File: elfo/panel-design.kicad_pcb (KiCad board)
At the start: 2 copper layers, 20 x 128.3 mm, 16 parts

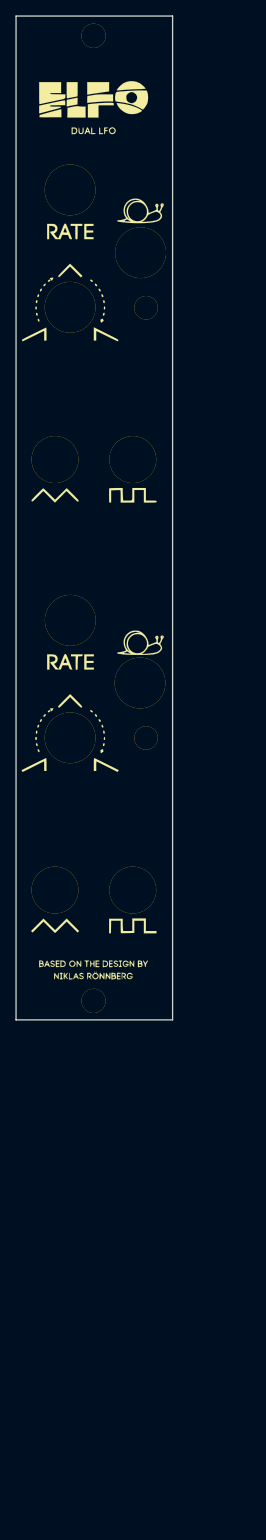
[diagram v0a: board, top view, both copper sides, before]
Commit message: Make ELFO nicer, fix issues
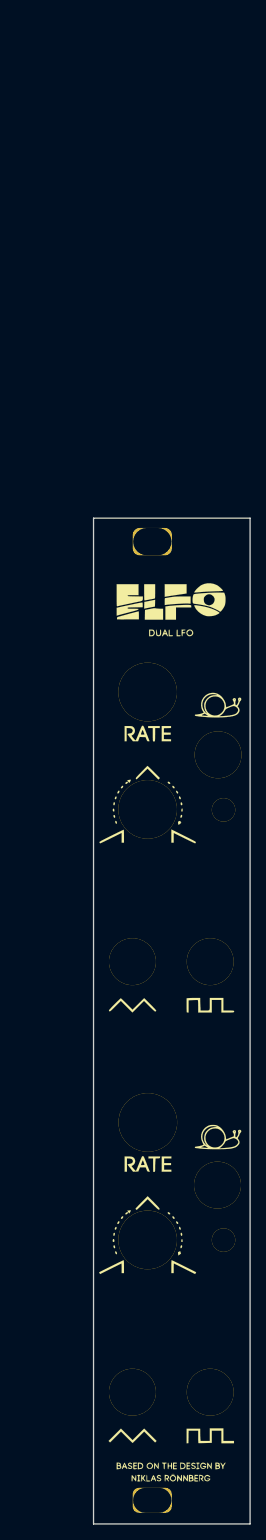
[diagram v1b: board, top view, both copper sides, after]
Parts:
- removed the ? at (-2.97, 13.1)
- removed the ? at (6.71, 28.1)
- removed the ? at (-4.93, 47.5)
- removed the ? at (5.01, 47.5)
- removed the ? at (0.00, -61.6)
- removed the ? at (0.00, 61.7)
- removed the ? at (5.01, -7.49)
- removed the ? at (-4.93, -7.49)
- removed the ? at (-2.99, -26.9)
- removed the ? at (6.01, -33.9)
- removed the ? at (6.71, -26.9)
- removed the ? at (-2.99, -41.9)
- removed the ? at (5.94, 21.1)
- removed the ? at (-2.99, 28.1)
- removed the G*** at (0.00, 0.00) (x2)
- added ?: , Wire_Pads:SolderWirePad_single_0-8mmDrill, F.Cu at (6.93, 77.2)
- added ?: , Wire_Pads:SolderWirePad_single_0-8mmDrill, F.Cu at (16.6, 92.2)
- added ?: , Wire_Pads:SolderWirePad_single_0-8mmDrill, F.Cu at (4.97, 111.7)
- added ?: , Wire_Pads:SolderWirePad_single_0-8mmDrill, F.Cu at (14.9, 111.7)
- added ?: , Wire_Pads:SolderWirePad_single_0-8mmDrill, F.Cu at (9.90, 2.52)
- added ?: , Wire_Pads:SolderWirePad_single_0-8mmDrill, F.Cu at (9.90, 125.0)
- added ?: , Wire_Pads:SolderWirePad_single_0-8mmDrill, F.Cu at (14.9, 56.7)
- added ?: , Wire_Pads:SolderWirePad_single_0-8mmDrill, F.Cu at (4.97, 56.7)
- added ?: , Wire_Pads:SolderWirePad_single_0-8mmDrill, F.Cu at (6.91, 37.2)
- added ?: , Wire_Pads:SolderWirePad_single_0-8mmDrill, F.Cu at (15.9, 30.2)
- added ?: , Wire_Pads:SolderWirePad_single_0-8mmDrill, F.Cu at (16.6, 37.3)
- added ?: , Wire_Pads:SolderWirePad_single_0-8mmDrill, F.Cu at (6.91, 22.2)
- added ?: , Wire_Pads:SolderWirePad_single_0-8mmDrill, F.Cu at (15.8, 85.2)
- added ?: , Wire_Pads:SolderWirePad_single_0-8mmDrill, F.Cu at (6.91, 92.2)
- added G***: LOGO, LOGO, F.Cu at (9.90, 64.2)
- added G***: LOGO, LOGO, F.Cu at (0.00, 0.00)
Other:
- board size 20 x 128.3 mm -> 20 x 128.5 mm
